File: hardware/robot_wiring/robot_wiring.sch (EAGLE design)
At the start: 124 parts

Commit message: galiper wirring : meca board added, need to update board version and final meca wirring
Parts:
- removed U$86, U$95, U$96, U$97, U$98: 1-794610-1, robotter_wiring:1-794610-1
- added U$143, U$144: 215083-4, robotter_wiring:215083-4
- added U$145, U$146: 08-50-0113, robotter_wiring:08-50-0113
- added U$155, U$156, U$157, U$158: 1-794610-1, robotter_wiring:1-794610-1
- added U$26: DC_MOTOR, robotter_wiring:DC_MOTOR
- added U$83: MOTOR_CTRL_PW_V3, robotter_wiring:MOTOR_CTRL_PW_V3
- added U$84: 1-2178712-6, robotter_wiring:1-2178712-6
- U$85: value 1-794610-1 -> 1-2178712-6; device robotter_wiring:1-794610-1 -> robotter_wiring:1-2178712-6
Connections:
- removed net N$15: BATTERY.-, U$101.P$1, U$28.P$1, U$30.P$1, U$90.P$1, U$93.P$1
- new net N$25: U$155.P$1, U$26.+
- new net N$26: U$156.P$1, U$26.-
- net GND: now also BATTERY.-, U$101.P$1, U$146.P$1, U$157.P$1, U$28.P$1, U$30.P$1, U$90.P$1, U$93.P$1
- net N$1: now also U$1.+; no longer U$97.P$1
- net N$2: now also U$1.-; no longer U$98.P$1
- net N$3: now also U$3.-; no longer U$86.P$1
- net N$4: now also U$3.+; no longer U$85.P$1
- net N$5: now also U$2.-; no longer U$96.P$1
- net N$6: now also U$2.+; no longer U$95.P$1
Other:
- note added: "MECA"

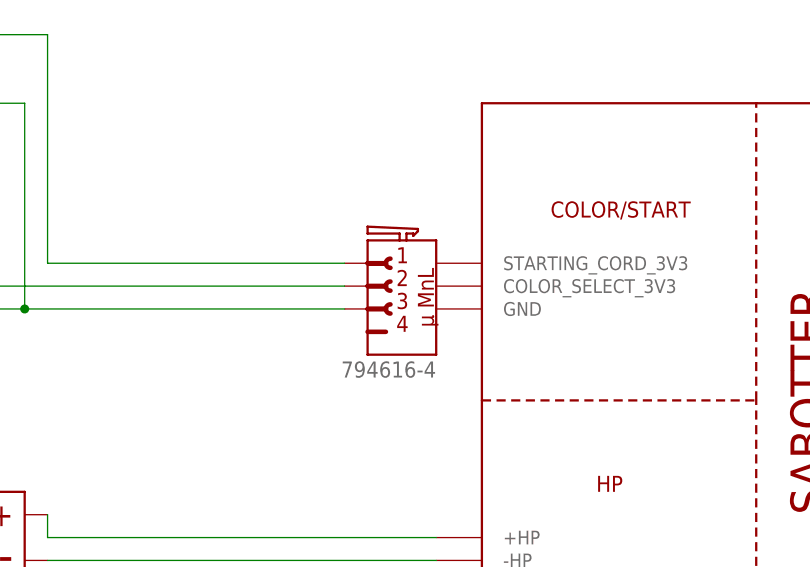
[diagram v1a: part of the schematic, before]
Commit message: robot schematic components updated
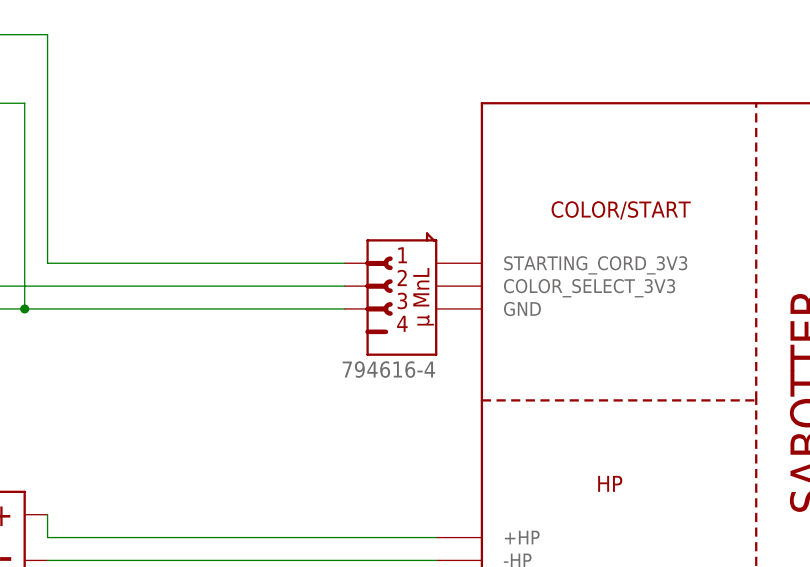
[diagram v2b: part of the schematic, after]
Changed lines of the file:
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@@
 <part name="U$104" library="robotter_wiring" deviceset="1-794610-1" device=""/>
 <part name="U$105" library="robotter_wiring" deviceset="1-794610-1" device=""/>
-<part name="U$106" library="robotter_wiring" deviceset="794616-4" device=""/>
 <part name="U$107" library="robotter_wiring" deviceset="51021-0500" device=""/>
 <part name="U$108" library="robotter_wiring" deviceset="51021-0500" device=""/>
@@
 <part name="U$84" library="robotter_wiring" deviceset="1-2178712-6" device=""/>
 <part name="U$85" library="robotter_wiring" deviceset="1-2178712-6" device=""/>
+<part name="U$86" library="robotter_wiring" deviceset="794616-4" device=""/>
 </parts>
 <sheets>
@@
 <instance part="U$104" gate="G$1" x="-304.8" y="-10.16" rot="R180"/>
 <instance part="U$105" gate="G$1" x="-304.8" y="-12.7" rot="R180"/>
-<instance part="U$106" gate="G$1" x="-297.18" y="-12.7" rot="MR0"/>
 <instance part="U$107" gate="G$1" x="27.94" y="73.66"/>
 <instance part="U$108" gate="G$1" x="78.74" y="78.74" rot="MR0"/>
@@
 <instance part="U$84" gate="G$1" x="-63.5" y="-236.22"/>
 <instance part="U$85" gate="G$1" x="-38.1" y="-236.22" rot="MR0"/>
+<instance part="U$86" gate="G$2" x="-297.18" y="-10.16"/>
 </instances>
 <busses>
